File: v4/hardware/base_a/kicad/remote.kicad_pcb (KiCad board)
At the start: 2 copper layers, 38.5 x 91.9 mm, 27 parts, among them J15 Conn_01x09_Female, J19 Conn_01x03_Female, J2 Conn_01x12_Female, J3 Conn_01x16_Female, J4 Conn_01x06_Female, J5 Conn_01x03_Female, J6 Conn_01x05_Female, Q1 Q_NMOS_GDS, Q3 Q_NPN_EBC, SW1 SW_Push, SW2 SW_Push, SW4 SW_Push_Dual, U1 RFM95HW

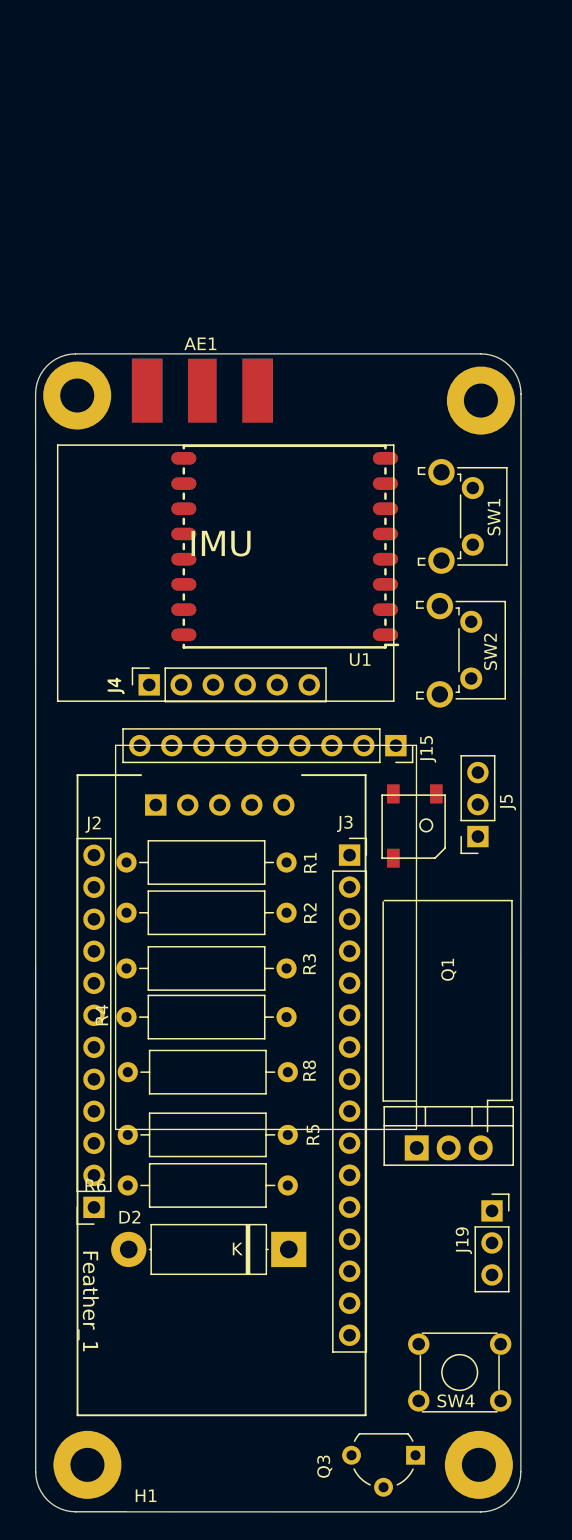
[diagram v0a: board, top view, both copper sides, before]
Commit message: basic layout
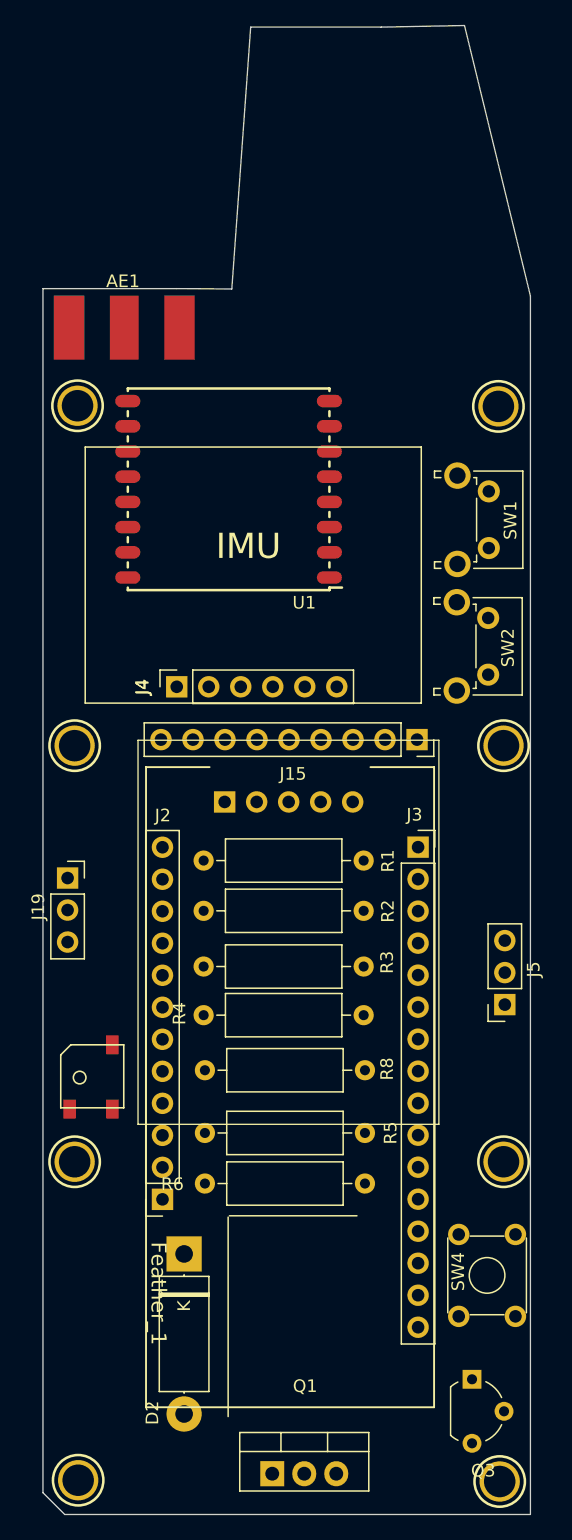
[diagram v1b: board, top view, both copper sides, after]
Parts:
- removed H1, H2, H5, H6: MountingHole_Pad, MountingHole:MountingHole_2.7mm_M2.5_Pad
- added H10: MountingHole, footprints:MOUNTINGHOLE_2.5_PLATED, F.Cu at (78.2, 131.9)
- added H11: MountingHole, footprints:MOUNTINGHOLE_2.5_PLATED, F.Cu at (78.1, 46.6)
- added H12: MountingHole, footprints:MOUNTINGHOLE_2.5_PLATED, F.Cu at (44.7, 46.5)
- added H3: MountingHole, footprints:MOUNTINGHOLE_2.5_PLATED, F.Cu at (44.5, 73.5)
- added H4: MountingHole, footprints:MOUNTINGHOLE_2.5_PLATED, F.Cu at (44.5, 106.5)
- added H7: MountingHole, footprints:MOUNTINGHOLE_2.5_PLATED, F.Cu at (78.5, 106.5)
- added H8: MountingHole, footprints:MOUNTINGHOLE_2.5_PLATED, F.Cu at (78.5, 73.5)
- added H9: MountingHole, footprints:MOUNTINGHOLE_2.5_PLATED, F.Cu at (44.7, 131.8)
- moved J19 42.8 mm to (43.9, 84.0)
- moved SP1 32.3 mm to (45.8, 99.7), turned to 90 degrees
- moved Q1 28.3 mm to (60.1, 131.3)
- moved J5 13.5 mm to (78.6, 94.0)
- moved D2 8.31 mm to (53.1, 113.8), turned to -90 degrees
- moved AE1 7.97 mm to (48.4, 37.8)
- moved Q3 7.51 mm to (76.0, 123.8), turned to -90 degrees
- moved SW4 7.49 mm to (74.9, 118.8), turned to 90 degrees
- moved U1 6.36 mm to (64.7, 60.1)
- moved R1 6.12 mm to (67.4, 82.6)
- moved R2 6.12 mm to (67.4, 86.6)
- moved R3 6.12 mm to (54.7, 91.0)
- moved R4 6.12 mm to (54.7, 94.9)
- moved R5 6.12 mm to (67.5, 104.2)
- moved R6 6.12 mm to (54.8, 108.2)
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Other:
- board size 38.5 x 91.9 mm -> 38.7 x 118.2 mm
